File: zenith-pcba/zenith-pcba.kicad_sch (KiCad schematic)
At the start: 0 parts

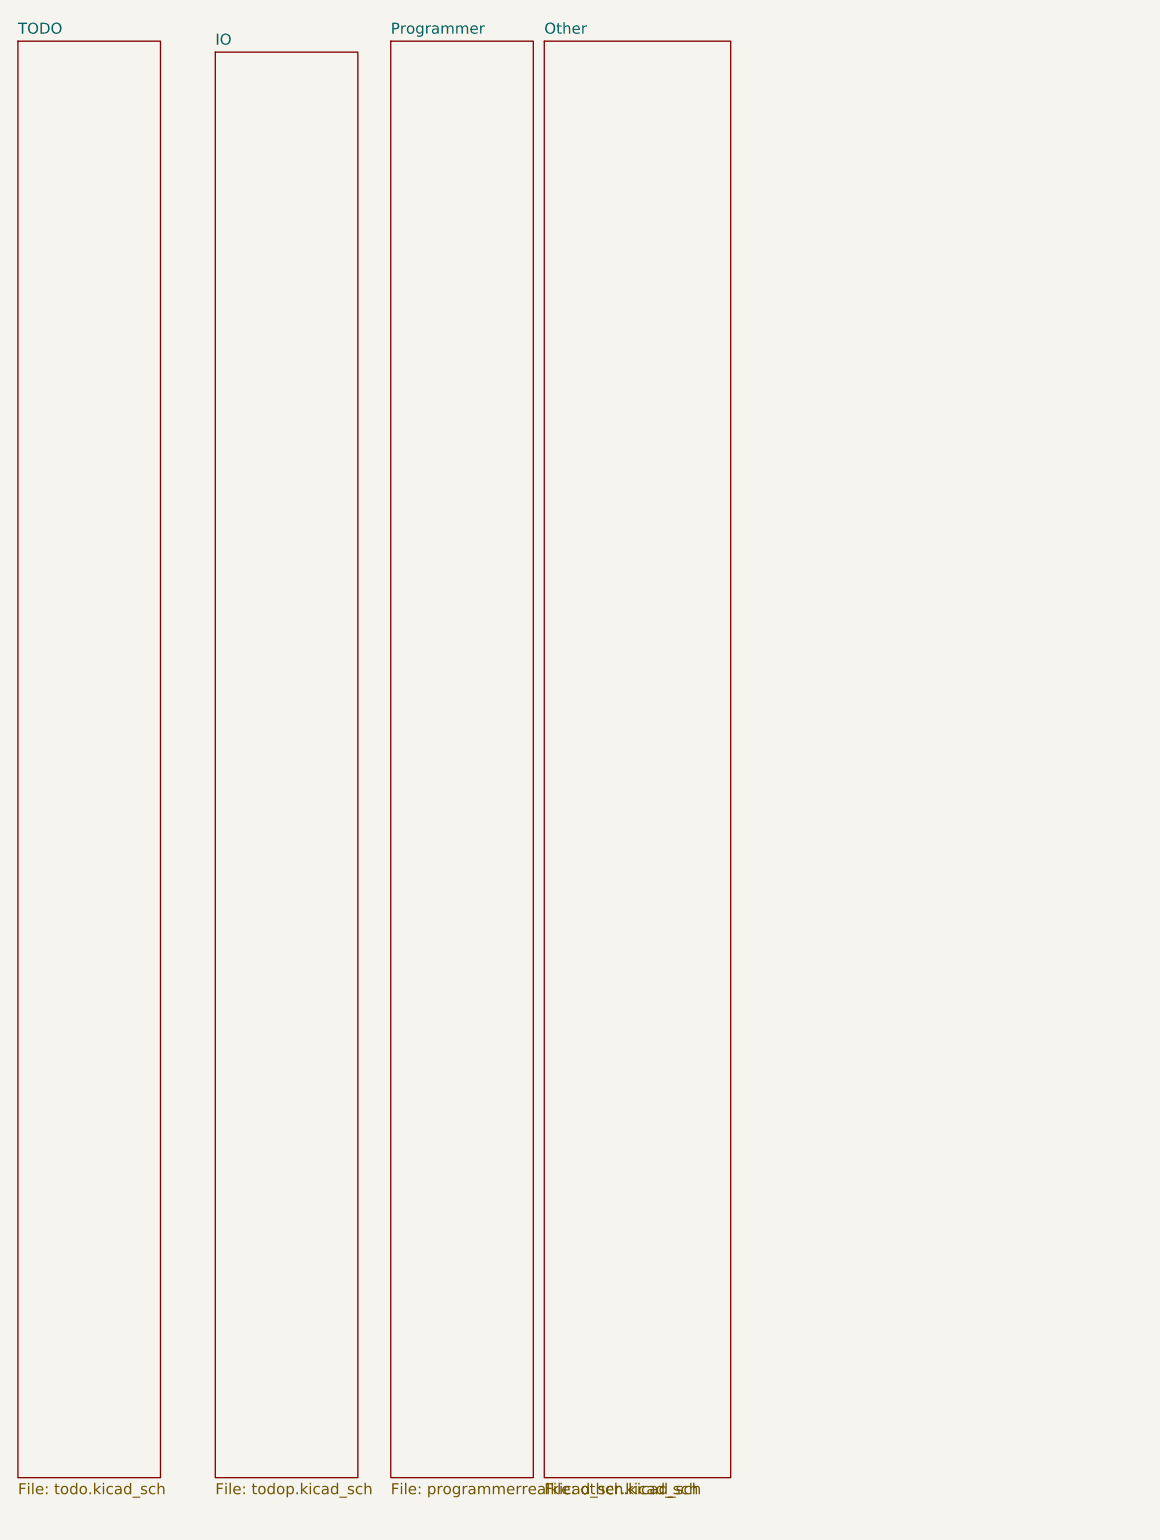
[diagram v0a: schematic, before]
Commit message: chore(pcba): clean up pages
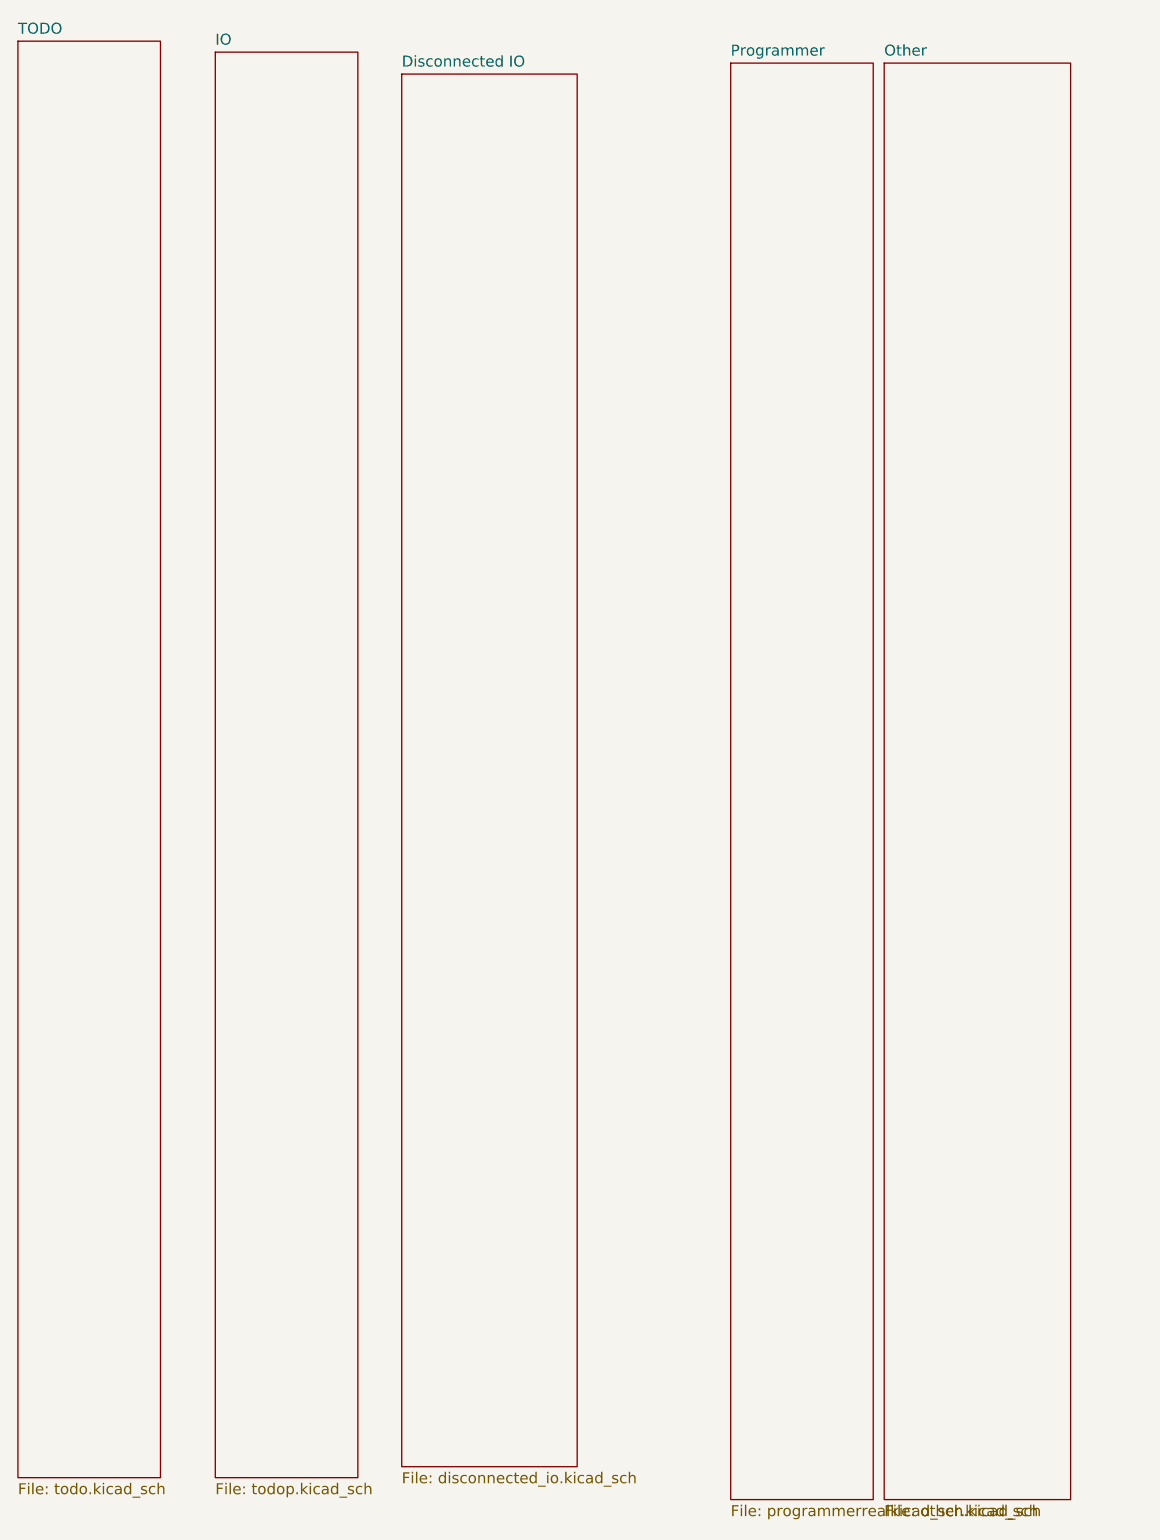
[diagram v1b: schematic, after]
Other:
- added sheet Disconnected IO (disconnected_io.kicad_sch)
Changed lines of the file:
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@@
 	(paper "A4")
 	(sheet
-		(at 82.55 20.32)
+		(at 66.04 24.13)
+		(size 20.32 161.29)
+		(exclude_from_sim no)
+		(in_bom yes)
+		(on_board yes)
+		(dnp no)
+		(fields_autoplaced yes)
+		(stroke
+			(width 0.1524)
+			(type solid)
+		)
+		(fill
+			(color 0 0 0 0)
+		)
+		(property "Sheetname" "Disconnected IO"
+			(at 66.04 23.4184 0)
+			(show_name no)
+			(do_not_autoplace no)
+			(effects
+				(font
+					(size 1.27 1.27)
+				)
+				(justify left bottom)
+			)
+		)
+		(property "Sheetfile" "disconnected_io.kicad_sch"
+			(at 66.04 186.0046 0)
+			(show_name no)
+			(do_not_autoplace no)
+			(effects
+				(font
+					(size 1.27 1.27)
+				)
+				(justify left top)
+			)
+		)
+		(instances
+			(project "zenith-pcba"
+				(path "/998c5703-2ef0-4484-8ced-1d53dcc65d39"
+					(page "4")
+				)
+			)
+		)
+	)
+	(sheet
+		(at 121.92 22.86)
 		(size 21.59 166.37)
 		(exclude_from_sim no)
@@
 		)
 		(property "Sheetname" "Other"
-			(at 82.55 19.6084 0)
+			(at 121.92 22.1484 0)
 			(show_name no)
 			(do_not_autoplace no)
@@
 		)
 		(property "Sheetfile" "other.kicad_sch"
-			(at 82.55 187.2746 0)
-			(show_name no)
-			(do_not_autoplace no)
-			(effects
-				(font
-					(size 1.27 1.27)
-				)
-				(justify left top)
-			)
-		)
-		(instances
-			(project "zenith-pcba"
-				(path "/998c5703-2ef0-4484-8ced-1d53dcc65d39"
-					(page "5")
+			(at 121.92 189.8146 0)
+			(show_name no)
+			(do_not_autoplace no)
+			(effects
+				(font
+					(size 1.27 1.27)
+				)
+				(justify left top)
+			)
+		)
+		(instances
+			(project "zenith-pcba"
+				(path "/998c5703-2ef0-4484-8ced-1d53dcc65d39"
+					(page "6")
 				)
 			)
@@
 	)
 	(sheet
-		(at 64.77 20.32)
+		(at 104.14 22.86)
 		(size 16.51 166.37)
 		(exclude_from_sim no)
@@
 		)
 		(property "Sheetname" "Programmer"
-			(at 64.77 19.6084 0)
+			(at 104.14 22.1484 0)
 			(show_name no)
 			(do_not_autoplace no)
@@
 		)
 		(property "Sheetfile" "programmerrealkicad_sch.kicad_sch"
-			(at 64.77 187.2746 0)
-			(show_name no)
-			(do_not_autoplace no)
-			(effects
-				(font
-					(size 1.27 1.27)
-				)
-				(justify left top)
-			)
-		)
-		(instances
-			(project "zenith-pcba"
-				(path "/998c5703-2ef0-4484-8ced-1d53dcc65d39"
-					(page "4")
-				)
-			)
+			(at 104.14 189.8146 0)
+			(show_name no)
+			(do_not_autoplace no)
+			(effects
+				(font
+					(size 1.27 1.27)
+				)
+				(justify left top)
+			)
+		)
+		(instances
+			(project "zenith-pcba"
+				(path "/998c5703-2ef0-4484-8ced-1d53dcc65d39"
+					(page "5")
+				)
+			)
